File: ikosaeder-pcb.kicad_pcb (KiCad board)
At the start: 2 copper layers, 21.9 x 20.8 mm, 5 parts, among them J1 Conn_01x03_Female, J2 Conn_01x03_Female, J3 Conn_01x03_Female, J4 Conn_01x03_Female, J5 Conn_01x03_Female

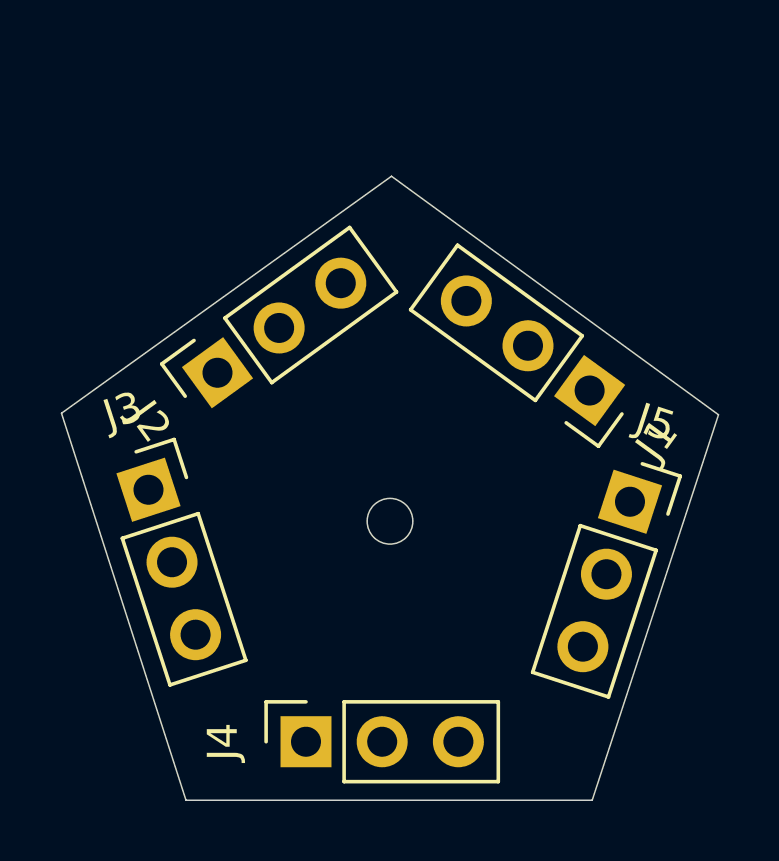
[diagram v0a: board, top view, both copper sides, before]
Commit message: Make the first pcb board which has the label A
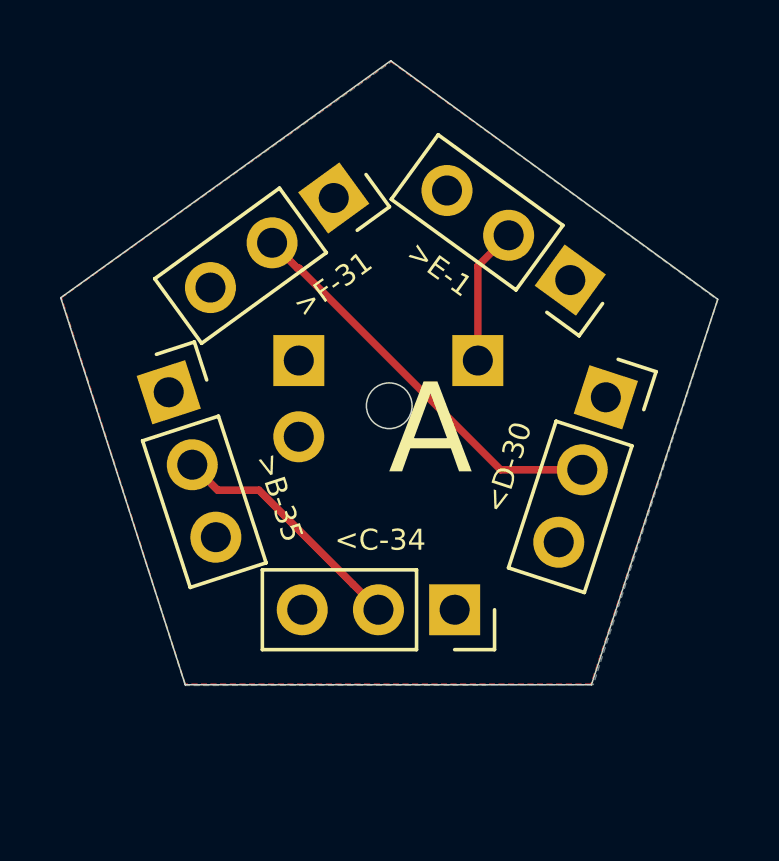
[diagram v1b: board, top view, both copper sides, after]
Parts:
- removed J1, J2, J3, J4, J5: Conn_01x03_Female, Connector_PinSocket_2.54mm:PinSocket_1x03_P2.54mm_Vertical
- added <C-34: Conn_01x03_Female, Connector_PinSocket_2.54mm:PinSocket_1x03_P2.54mm_Vertical, F.Cu at (109.0, 93.7)
- added <D-30: Conn_01x03_Female, Connector_PinSocket_2.54mm:PinSocket_1x03_P2.54mm_Vertical, F.Cu at (114.0, 86.6)
- added >B-35: Conn_01x03_Female, Connector_PinSocket_2.54mm:PinSocket_1x03_P2.54mm_Vertical, F.Cu at (99.4, 86.4)
- added >E-1: Conn_01x03_Female, Connector_PinSocket_2.54mm:PinSocket_1x03_P2.54mm_Vertical, F.Cu at (112.8, 82.7)
- added >F-31: Conn_01x03_Female, Connector_PinSocket_2.54mm:PinSocket_1x03_P2.54mm_Vertical, F.Cu at (104.9, 79.9)
- added Power1: Conn_01x02_Female, Connector_PinHeader_2.54mm:PinHeader_1x02_P2.54mm_Vertical, B.Cu at (103.8, 85.3)
- added Signal1: Conn_01x01_Female, Connector_PinHeader_2.54mm:PinHeader_1x01_P2.54mm_Vertical, B.Cu at (109.7, 85.3)
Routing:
- net Net-(<D-30-Pad2): track 0.00 -> 13.5 mm
- net Net-(<C-34-Pad2): track 0.00 -> 8.21 mm
- net Net-(>E-1-Pad2): track 0.00 -> 4.60 mm
- added copper zone on B.Cu, net +5V
- added copper zone on F.Cu, net GND
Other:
- outline, holes or cut-outs redrawn
- board text added: "5V"
- board text added: "A"
- board text added: "GND"
